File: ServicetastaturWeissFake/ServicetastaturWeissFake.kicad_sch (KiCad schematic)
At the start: 68 parts, among them J1 Automat, SW1 Gewinn, SW10 Lautspr./, SW11 ↓0,10, SW12 ↑0,10, SW13 ↓Serie, SW14 ↑Serie, SW15 Zeit, SW16 ↑1,-, SW17 ↙0,10, SW18 ↙1,-, SW19 Auszahlquote, SW2 Foul, SW20 ↙5,-, SW21 Münzsp., SW22 Sp.Zähl, SW23 Lampen, SW24 Reset, SW25 Initialisieren, SW26 Münzung, SW27 Ende, SW28 ↑0,10, SW29 ↓Serie, SW3 ↙2,-, SW30 ↑Serie, SW31 ↓1,-, SW32 ↑1,-, SW4 HW-Test, SW5 Münzsp., SW6 Sp.Zähl, SW7 Dauerlauf, SW8 Reset, SW9 Initialisieren, U1 CC56-12CGKWA, U2 CC56-12CGKWA, U3 74LS48, U4 74LS145, U5 74LS48, U6 74LS145

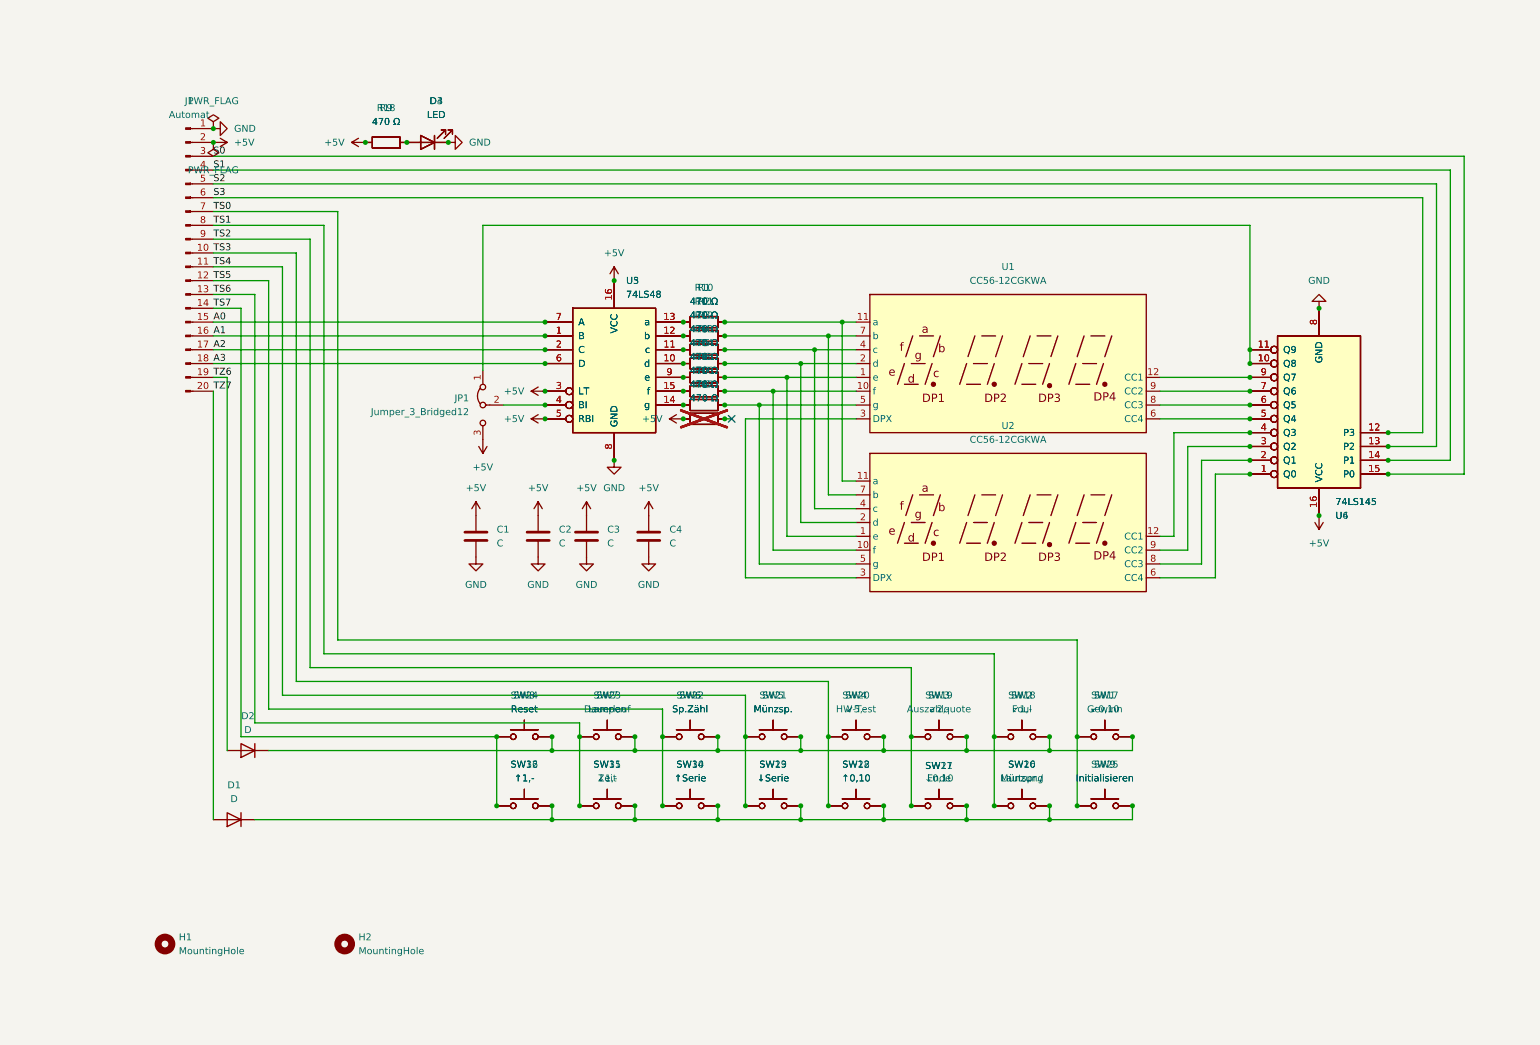
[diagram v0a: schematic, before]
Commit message: schaltplan
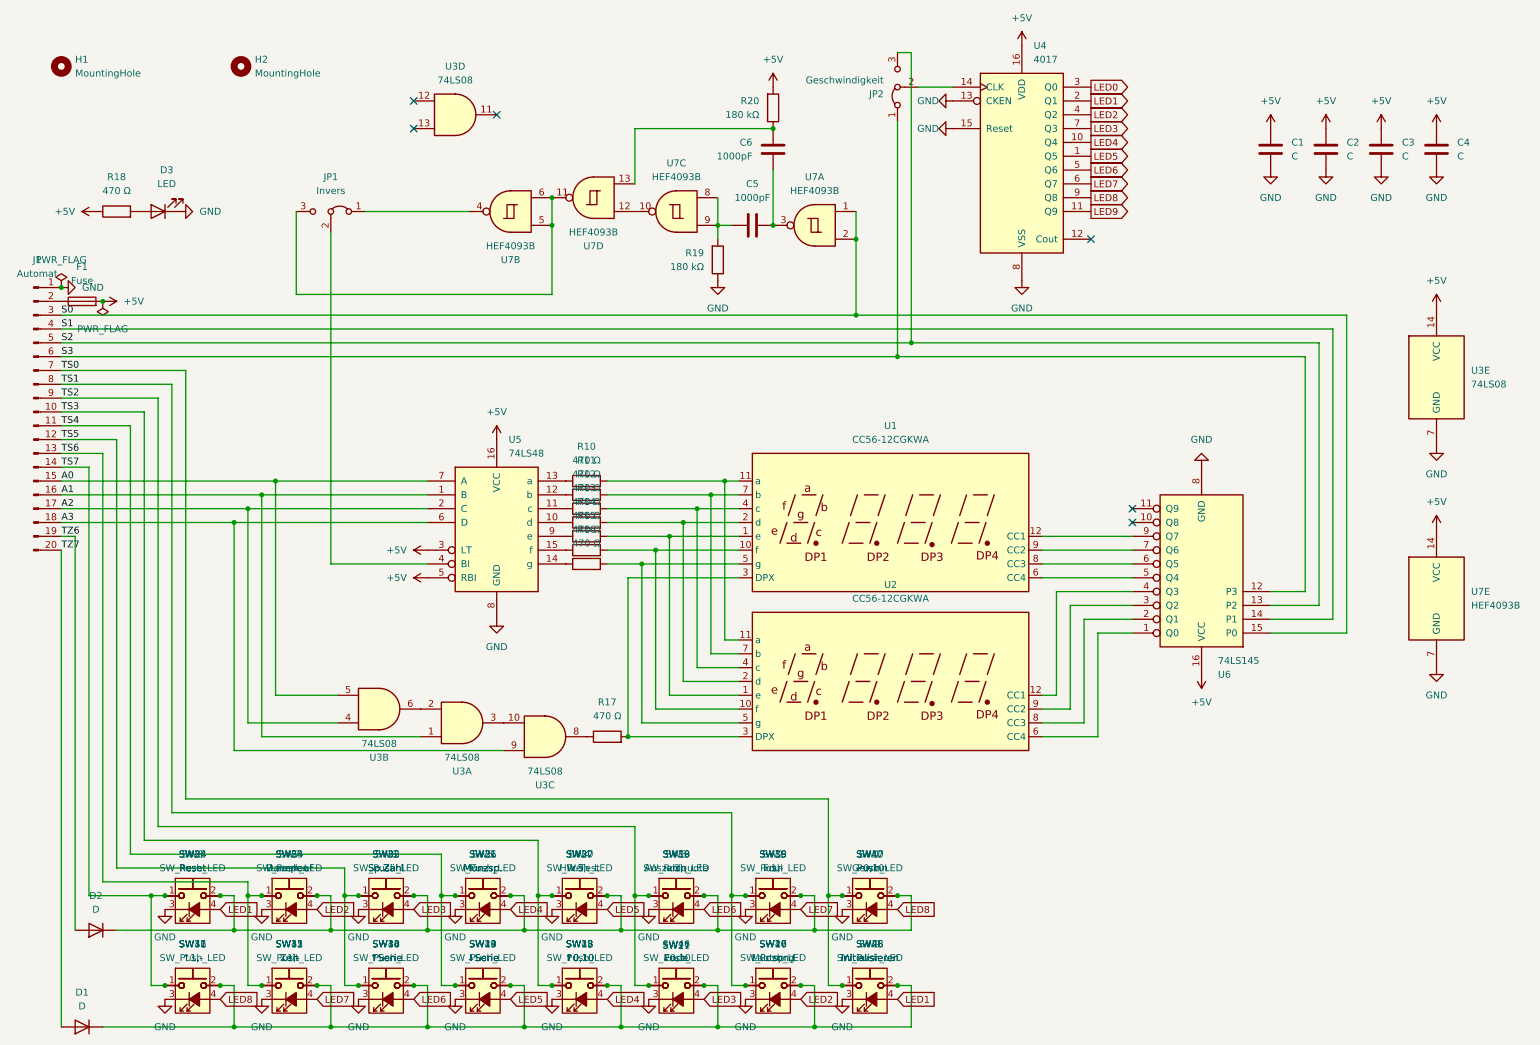
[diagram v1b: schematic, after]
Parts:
- removed D4: LED, LED_SMD:LED_0805_2012Metric, symbol Device:LED
- removed R1, R2, R3, R4, R5, R6, R7, R8, R9: 470 Ω, Resistor_THT:R_Axial_DIN0207_L6.3mm_D2.5mm_P7.62mm_Horizontal, symbol Device:R
- removed U3: 74LS48, Package_DIP:DIP-16_W7.62mm, symbol 74xx:74LS48
- removed U4: 74LS145, Package_DIP:DIP-16_W7.62mm, symbol 74xx:74LS145
- added C5, C6: 1000pF, Capacitor_SMD:C_0603_1608Metric, symbol Device:C
- added F1: Fuse, Fuse:Fuse_0805_2012Metric, symbol Device:Fuse
- added JP2: Geschwindigkeit, Jumper:SolderJumper-3_P1.3mm_Bridged12_Pad1.0x1.5mm, symbol Jumper:Jumper_3_Bridged12
- added R19, R20: 180 kΩ, Resistor_SMD:R_0603_1608Metric, symbol Device:R
- added SW33, SW34, SW35, SW36, SW37, SW38, SW39, SW40, SW41, SW42, SW43, SW44, SW45, SW46, SW47, SW48: SW_Push_LED, symbol Switch:SW_Push_LED
- added U3: 74LS08, Package_SO:SOIC-14_3.9x8.7mm_P1.27mm, symbol 74xx:74LS08
- added U4: 4017, Package_SO:SOP-16_3.9x9.9mm_P1.27mm, symbol 4xxx:4017
- added U7: HEF4093B, Package_SO:SOIC-14_3.9x8.7mm_P1.27mm, symbol 4xxx:HEF4093B
- C3, C4: footprint Capacitor_SMD:C_0805_2012Metric -> Capacitor_SMD:C_0603_1608Metric
- JP1: value Jumper_3_Bridged12 -> Invers; footprint Jumper:SolderJumper-3_P1.3mm_Bridged12_Pad1.0x1.5mm_NumberLabels -> Jumper:SolderJumper-3_P1.3mm_Bridged12_Pad1.0x1.5mm
- R10, R11, R12, R13, R14, R15, R16, R18: footprint Resistor_SMD:R_0805_2012Metric -> Resistor_SMD:R_0603_1608Metric
- R17: footprint Resistor_SMD:R_0805_2012Metric -> Resistor_SMD:R_0603_1608Metric; now fitted
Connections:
- net +5V: now also F1.2, R20.2, U3.14 (VCC), U4.16 (VDD), U7.14 (VCC); no longer J1.2 (Pin_2), JP1.3 (B), R17.1
- net A0: now also U3.5
- net A1: now also U3.1
- net A2: now also U3.4
- net A3: now also U3.9
- net GND: now also R19.1, SW33.3 (K), SW34.3 (K), SW35.3 (K), SW37.3 (K), SW38.3 (K), SW39.3 (K), SW40.3 (K), SW41.3 (K), SW42.3 (K), SW43.3 (K), SW44.3 (K), SW45.3 (K), SW46.3 (K), SW47.3 (K), SW48.3 (K), U3.7 (GND), U4.13 (CKEN), U4.15 (Reset), U4.8 (VSS), U7.7 (GND)
- net S0: now also U7.1, U7.2
- net S2: now also JP2.3 (B)
- net S3: now also JP2.1 (A)
- net TS0: now also SW40.1, SW48.1
- net TS1: now also SW39.1, SW47.1
- net TS2: now also SW38.1, SW46.1
- net TS3: now also SW37.1, SW45.1
- net TS4: now also SW36.1, SW44.1
- net TS5: now also SW35.1, SW43.1
- net TS6: now also SW34.1, SW42.1
- net TS7: now also SW33.1, SW41.1
- net at D1.1 (K), SW10.1, SW11.1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: now also SW41.2, SW42.2, SW43.2, SW44.2, SW45.2, SW46.2, SW47.2, SW48.2
- net at U1.3 (DPX), U2.3 (DPX): now also R17.2
- net at D2.1 (K), SW1.1, SW17.1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: now also SW33.2, SW34.2, SW35.2, SW36.2, SW37.2, SW38.2, SW39.2, SW40.2
- new net: U7.10, U7.12
- new net: C5.2, R19.2, U7.8, U7.9
- new net: R17.1, U3.8
- new net: U3.2, U3.6
- new net: U3.10, U3.3
- new net: JP1.1 (A), U7.4
- new net: JP1.3 (B), U7.11, U7.5, U7.6
- new net: C6.2, R20.1, U7.13
- new net: F1.1, J1.2 (Pin_2)
- new net: JP2.2 (C), U4.14 (CLK)
- new net: C5.1, C6.1, U7.3
- new net LED0: U4.3 (Q0)
- new net LED1: SW33.4 (A), SW48.4 (A), U4.2 (Q1)
- new net LED2: SW34.4 (A), SW47.4 (A), U4.4 (Q2)
- new net LED3: SW35.4 (A), SW46.4 (A), U4.7 (Q3)
- new net LED4: SW36.4 (A), SW45.4 (A), U4.10 (Q4)
- new net LED5: SW37.4 (A), SW44.4 (A), U4.1 (Q5)
- new net LED6: SW38.4 (A), SW43.4 (A), U4.5 (Q6)
- new net LED7: SW39.4 (A), SW42.4 (A), U4.6 (Q7)
- new net LED8: SW40.4 (A), SW41.4 (A), U4.9 (Q8)
- new net LED9: U4.11 (Q9)
- now unconnected: U6.10 (Q8), U6.11 (Q9)
- no-connect marks 1 -> 6
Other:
- moved on the sheet: C1, C2, C3, C4, D1, D2, D3, H1, H2, J1, R10, R11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
